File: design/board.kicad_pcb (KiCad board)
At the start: 2 copper layers, 39.4 x 29.2 mm, 14 parts, among them J1 Barrel_Jack_Switch, J2 Conn_01x01_Male, J3 Conn_01x01_Male, J4 Conn_01x01_Male, J5 Conn_01x01_Male, SW1 main

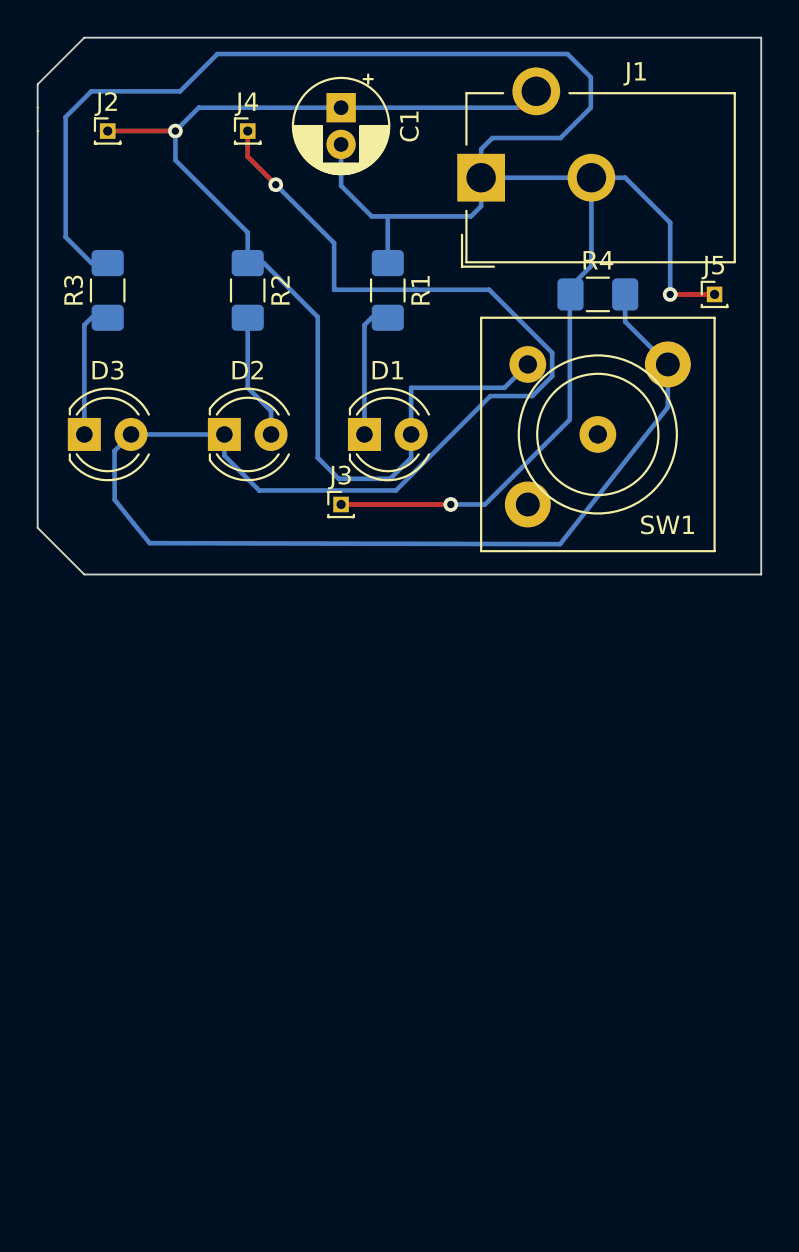
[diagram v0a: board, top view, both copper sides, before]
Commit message: New pcb design.
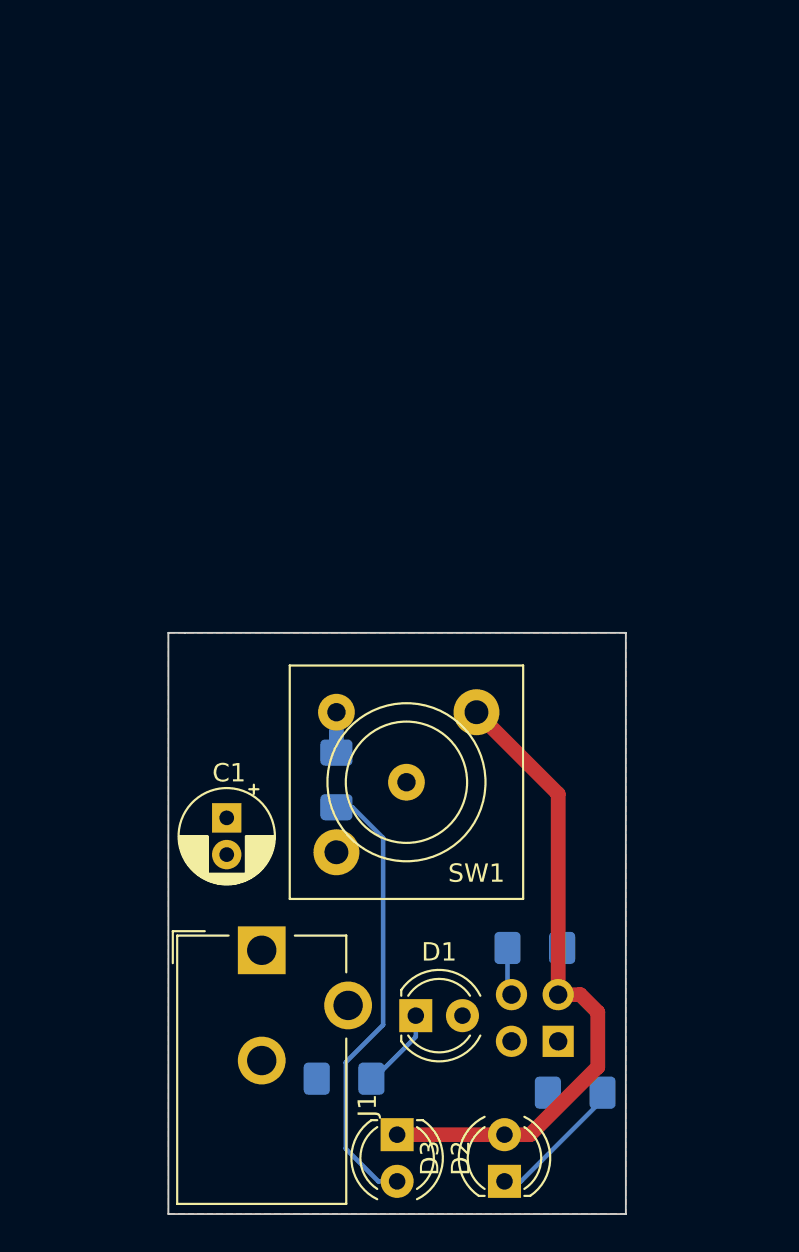
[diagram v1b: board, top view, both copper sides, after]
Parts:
- removed J2, J3, J4, J5: Conn_01x01_Male, Connector_PinHeader_1.00mm:PinHeader_1x01_P1.00mm_Vertical
- added J6: Conn_01x04_Female, Connector_PinSocket_2.54mm:PinSocket_2x02_P2.54mm_Vertical, B.Cu at (182.0, 90.2)
- R1, R2, R3, R4: moved to B.Cu
- moved R3 50.5 mm to (182.9, 93.0), turned to 180 degrees
- moved D3 46.6 mm to (179.1, 97.8), turned to 90 degrees
- moved J1 43.7 mm to (165.9, 85.2), turned to 0 degrees
- moved R1 43.0 mm to (170.3, 92.2), turned to 0 degrees
- moved D2 39.2 mm to (173.2, 95.2), turned to 270 degrees
- moved C1 39.1 mm to (164.0, 78.0)
- moved R4 35.7 mm to (180.7, 85.1)
- moved D1 31.7 mm to (174.2, 88.8)
- moved R2 27.1 mm to (169.9, 75.9)
- moved SW1 21.6 mm to (173.7, 68.5)
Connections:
- net /+5V renamed /VCC_OUT
- net Net-(D1-Pad1) renamed /MID_PWR
- net Net-(D2-Pad2) renamed /MID_OFF
- net Net-(D3-Pad1) renamed /MID_ON
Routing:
- net GND: track 110.5 -> 2.63 mm, vias 2 -> 0
- net /VCC_OUT: track 98.4 -> 37.8 mm, vias 1 -> 0
- net VCC: track 62.4 -> 2.20 mm, vias 1 -> 0
- net /MID_OFF: track 6.88 -> 24.5 mm
- net /MID_PWR: track 7.39 -> 4.51 mm
- added copper zone on B.Cu, net GND
- added copper zone on F.Cu, net VCC
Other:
- board size 39.4 x 29.2 mm -> 24.9 x 31.6 mm
